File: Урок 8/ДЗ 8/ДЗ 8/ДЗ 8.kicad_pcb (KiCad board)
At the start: 2 copper layers, 63.5 x 70.5 mm, 29 parts, among them K1 HONGFA_HFD2-0xx-x-L2-x, K2 HONGFA_HFD2-0xx-x-L2-x, SW1 SW_Push, SW2 SW_Push

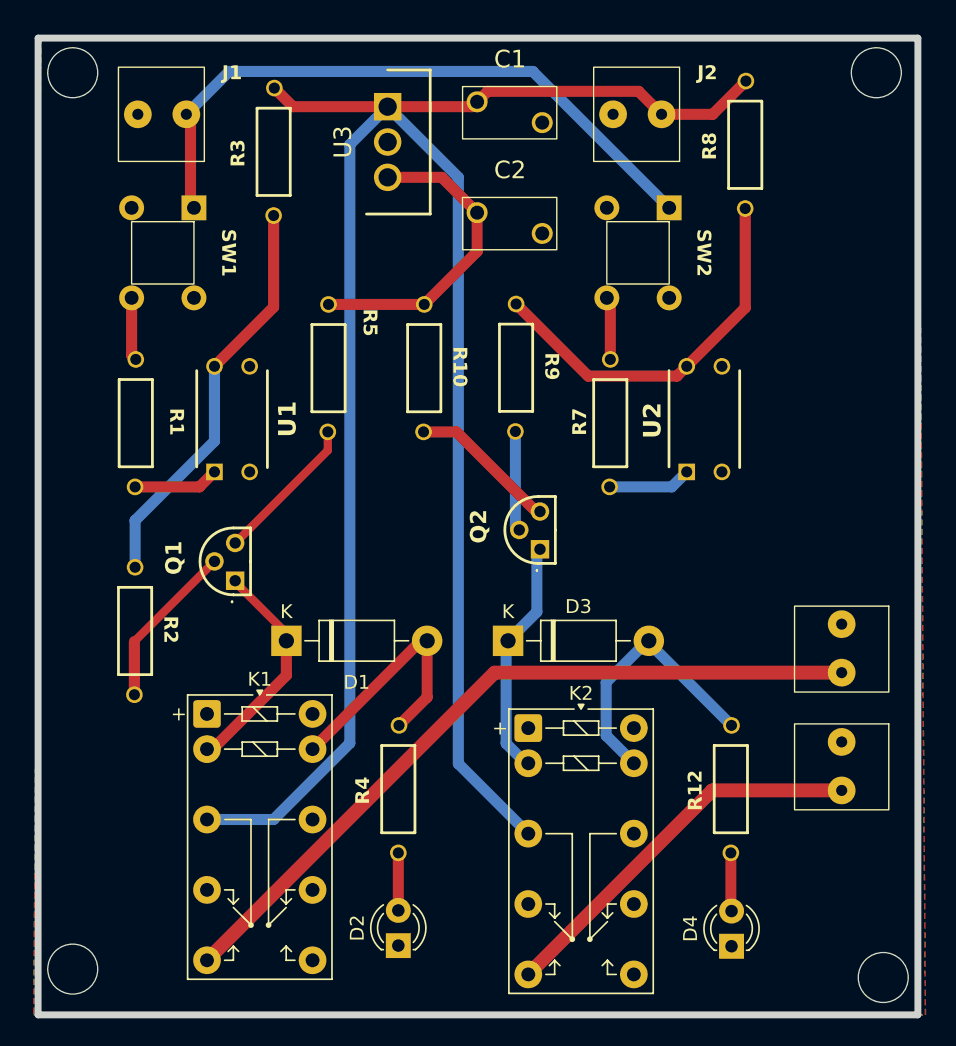
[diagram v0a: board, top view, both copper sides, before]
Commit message: 1
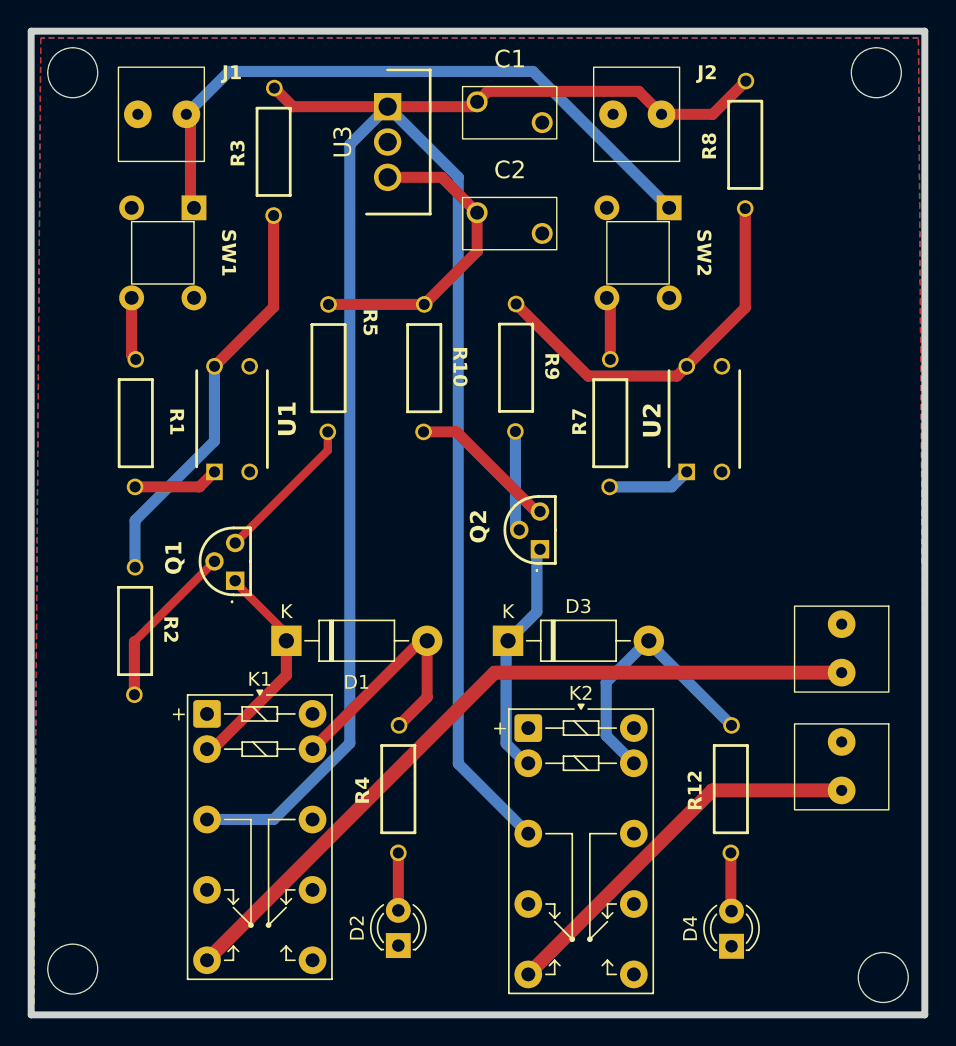
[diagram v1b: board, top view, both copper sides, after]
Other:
- board size 63.5 x 70.5 mm -> 64.5 x 71 mm
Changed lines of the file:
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@@
 	)
 	(gr_rect
-		(start 46 24.5)
-		(end 109.5 95)
+		(start 45.5 24)
+		(end 110 95)
 		(stroke
 			(width 0.5)
@@
 		(min_thickness 0.25)
 		(filled_areas_thickness no)
-		(fill
+		(fill yes
 			(thermal_gap 0.5)
 			(thermal_bridge_width 0.5)
